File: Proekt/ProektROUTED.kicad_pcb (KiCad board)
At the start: 2 copper layers, 40 x 40 mm, 36 parts, among them J1 RGB, J2 LX, J3 I2C, J4 UART, J5 USB_C_USB2.0, Q1 TEPT5700, SW1 RST, SW2 BTN, U1 ESP32-C3, U2 R1170H331B, U3 USBLC6-2SC6

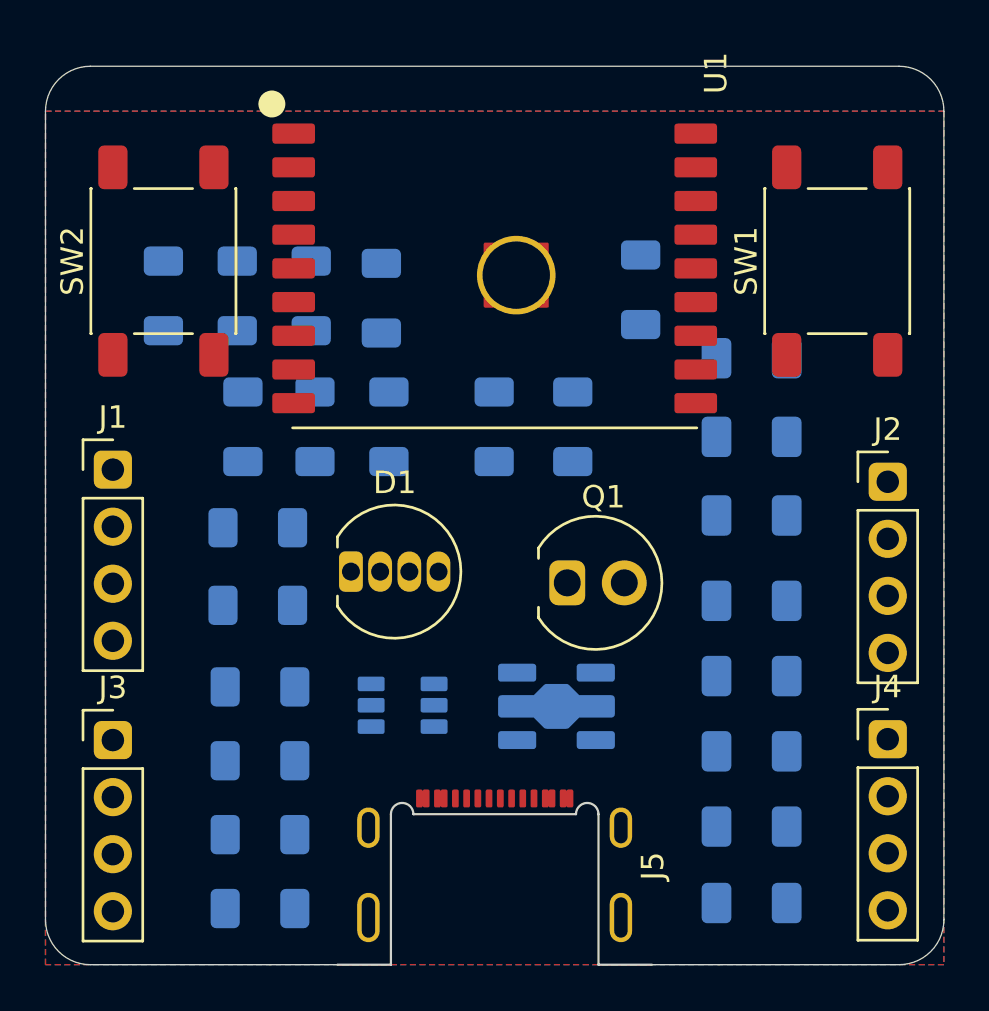
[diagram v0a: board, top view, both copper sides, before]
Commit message: dodadeno pcb design
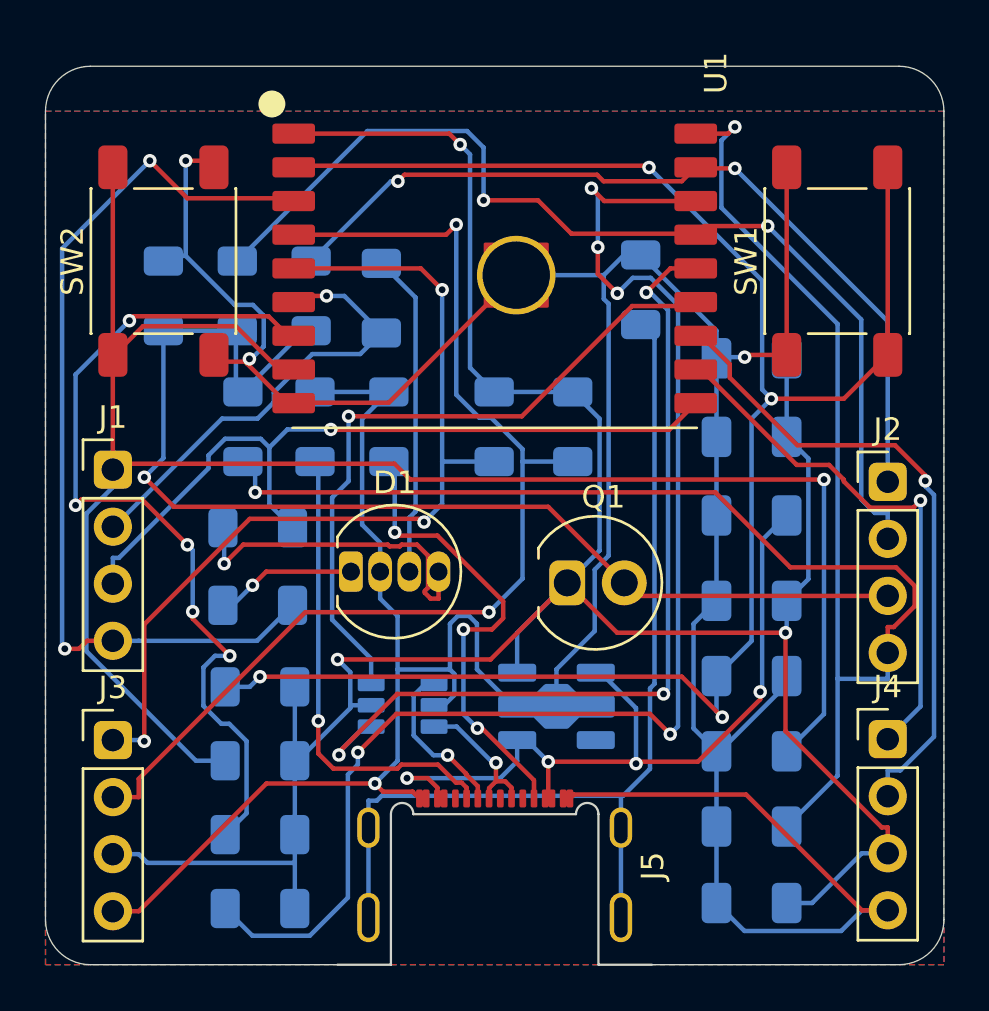
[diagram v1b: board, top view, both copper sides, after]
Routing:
- net GND: track 0.00 -> 189.7 mm, vias 0 -> 4
- net +3.3V: track 0.00 -> 114.8 mm, vias 0 -> 3
- net BTN: track 0.00 -> 84.5 mm, vias 0 -> 1
- net Net-(U1-EN): track 0.00 -> 81.1 mm, vias 0 -> 4
- net LX_OUT: track 0.00 -> 76.1 mm, vias 0 -> 2
- net Net-(U1-IO2/ADC1_2/FSPIQ): track 0.00 -> 61.1 mm, vias 0 -> 5
- net LX_C: track 0.00 -> 52.5 mm, vias 0 -> 1
- net SDA: track 0.00 -> 49.7 mm, vias 0 -> 2
- net LX_B: track 0.00 -> 45.9 mm, vias 0 -> 2
- net Net-(J5-CASE): track 0.00 -> 43.9 mm
- net LED_B: track 0.00 -> 41.5 mm, vias 0 -> 2
- net SCL: track 0.00 -> 41.1 mm, vias 0 -> 3
- net Net-(U1-IO8): track 0.00 -> 38.8 mm, vias 0 -> 5
- net USB_D+: track 0.00 -> 38.8 mm, vias 0 -> 3
- net LX_A: track 0.00 -> 37.6 mm, vias 0 -> 2
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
